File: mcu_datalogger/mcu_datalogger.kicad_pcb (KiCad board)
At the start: 2 copper layers, 51.9 x 31.1 mm, 29 parts, among them J1 Conn_01x04_Pin, J2 Conn_01x04_Pin, J3 Conn_01x09, J4 Conn_02x03_Odd_Even, U1 24LC1025, U2 24LC1025, U3 DS1337S_, U4 ATMEGA328P-AU, Y1 16 MHz, Y2 32.768KHz

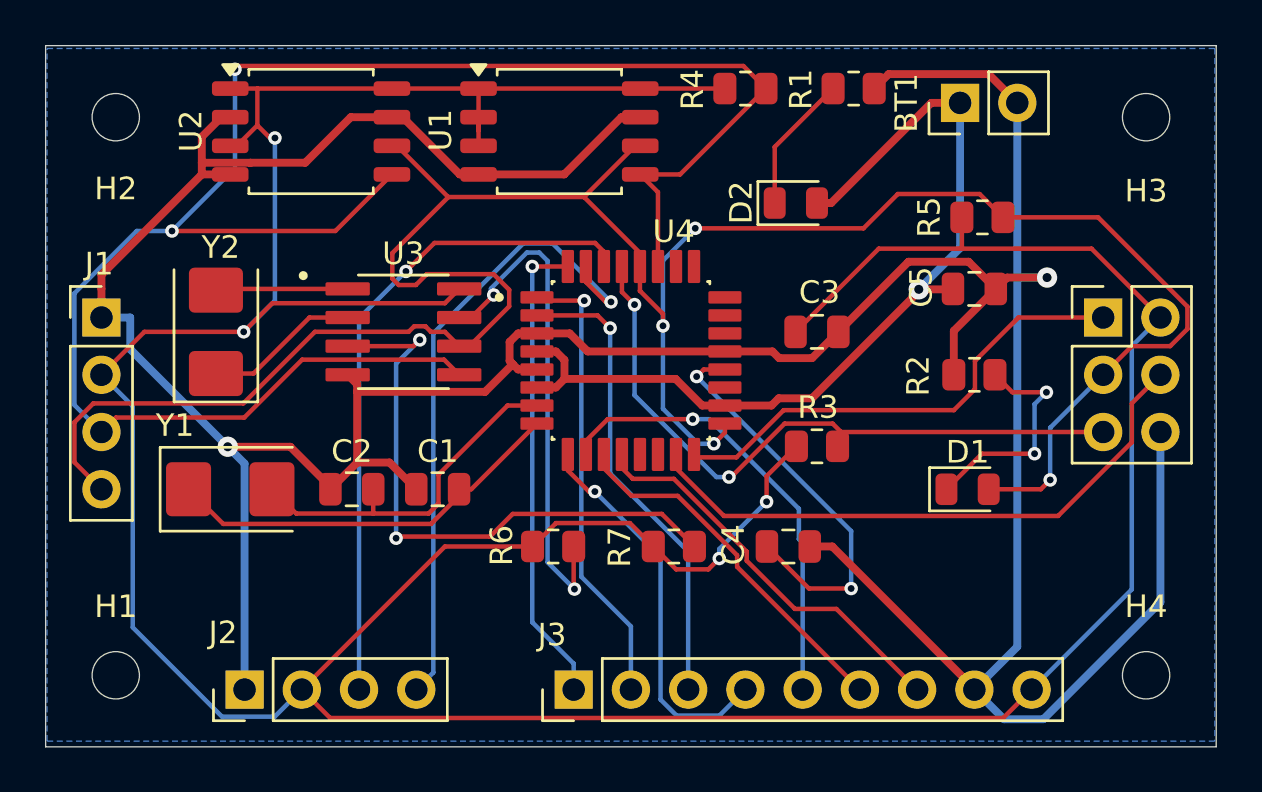
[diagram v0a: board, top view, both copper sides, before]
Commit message: back copper vias
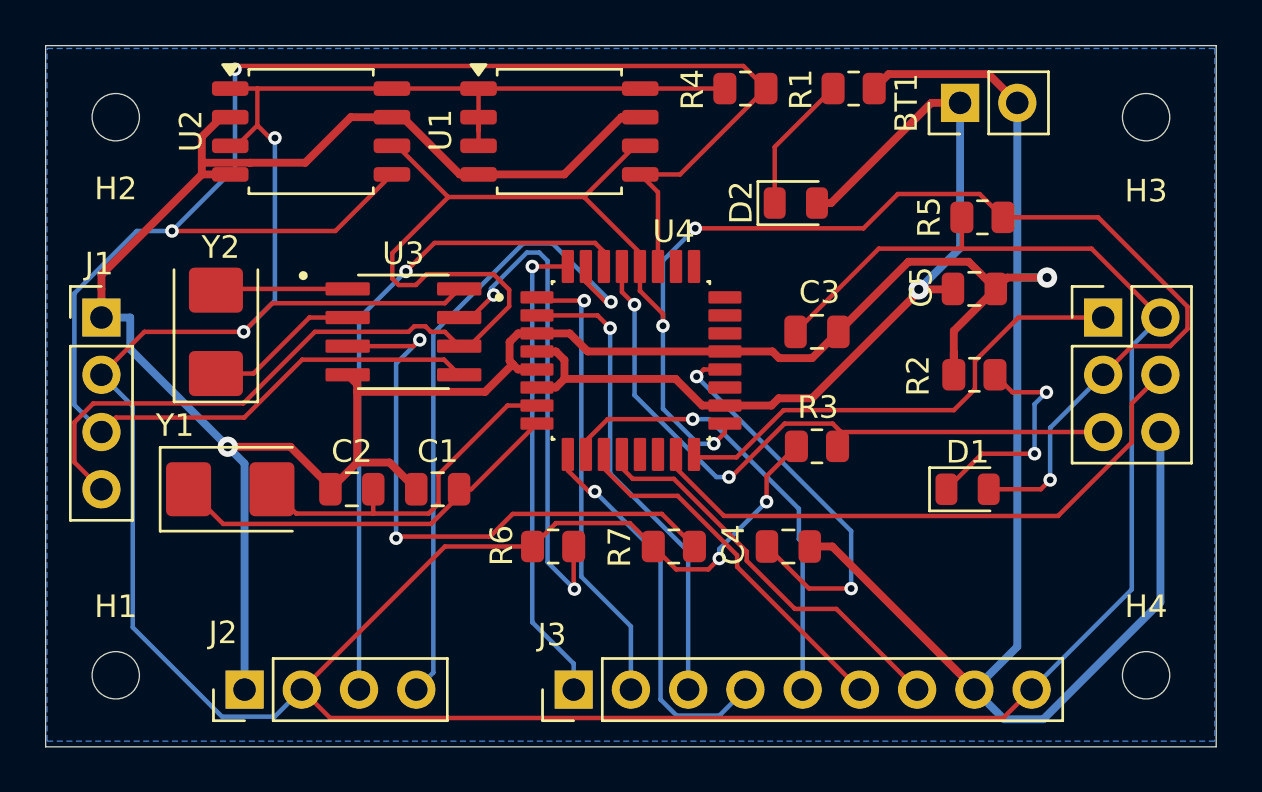
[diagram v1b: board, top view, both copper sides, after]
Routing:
- net GND: track 174.2 -> 175.1 mm
- net Net-(D1-K): track 10.1 -> 10.7 mm
